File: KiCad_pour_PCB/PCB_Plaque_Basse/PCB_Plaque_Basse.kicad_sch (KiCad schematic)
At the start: 9 parts

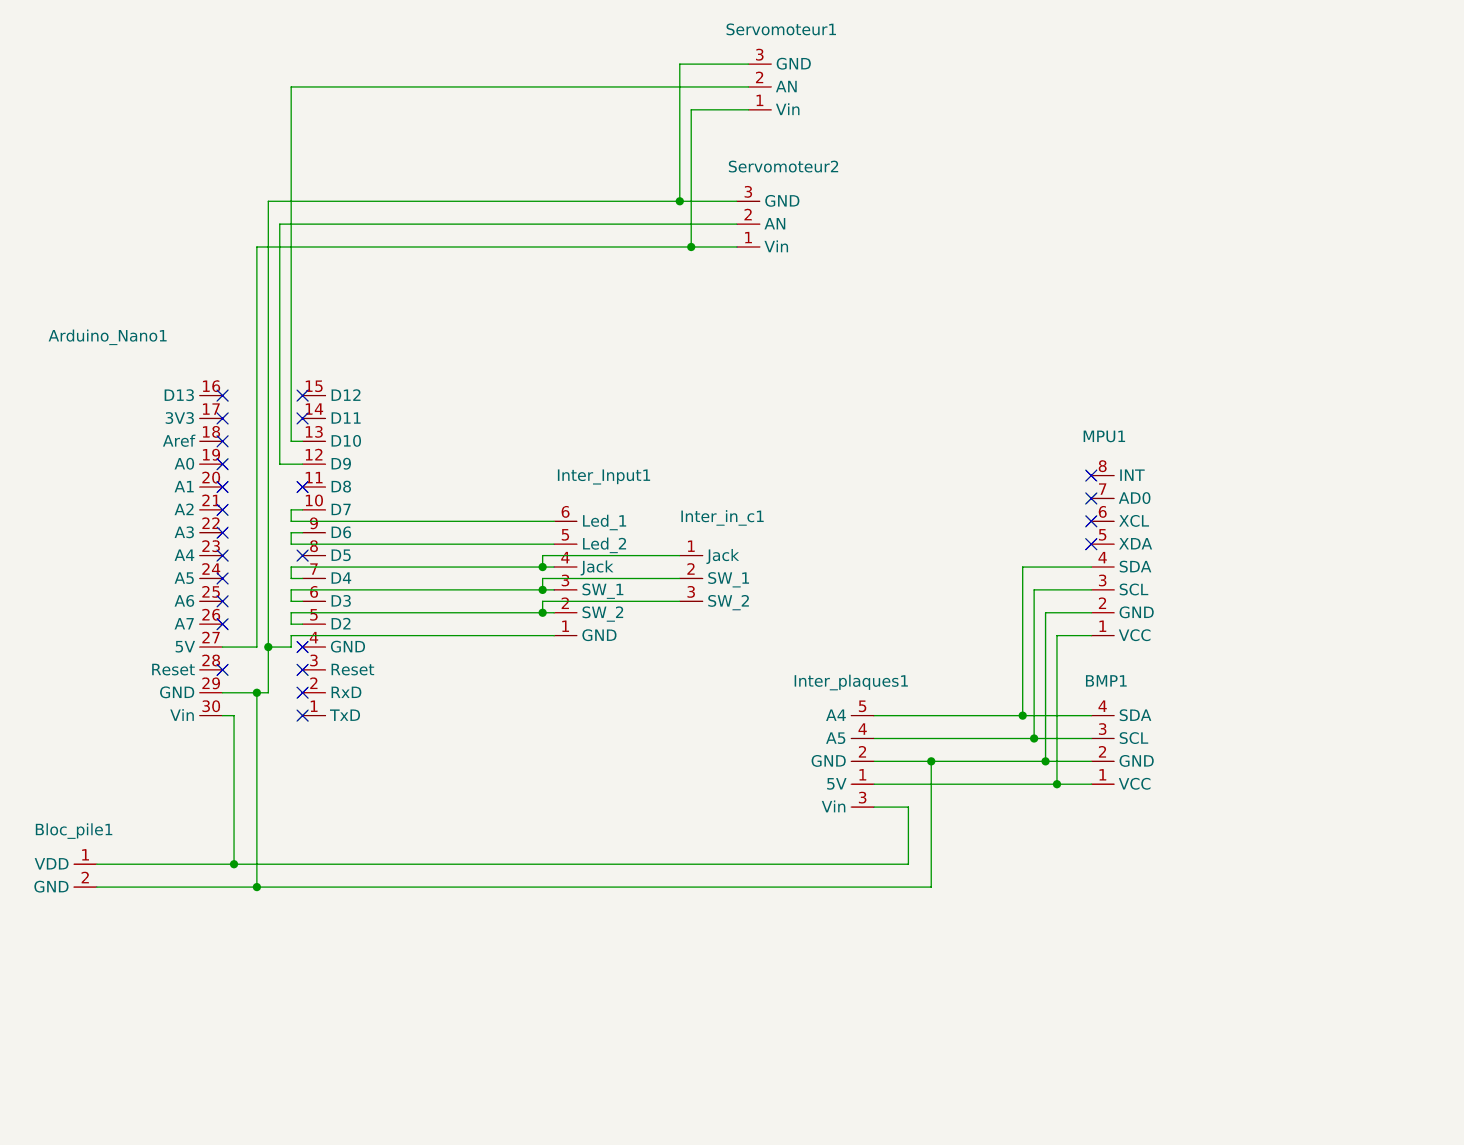
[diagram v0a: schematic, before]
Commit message: Avancement carte PCB
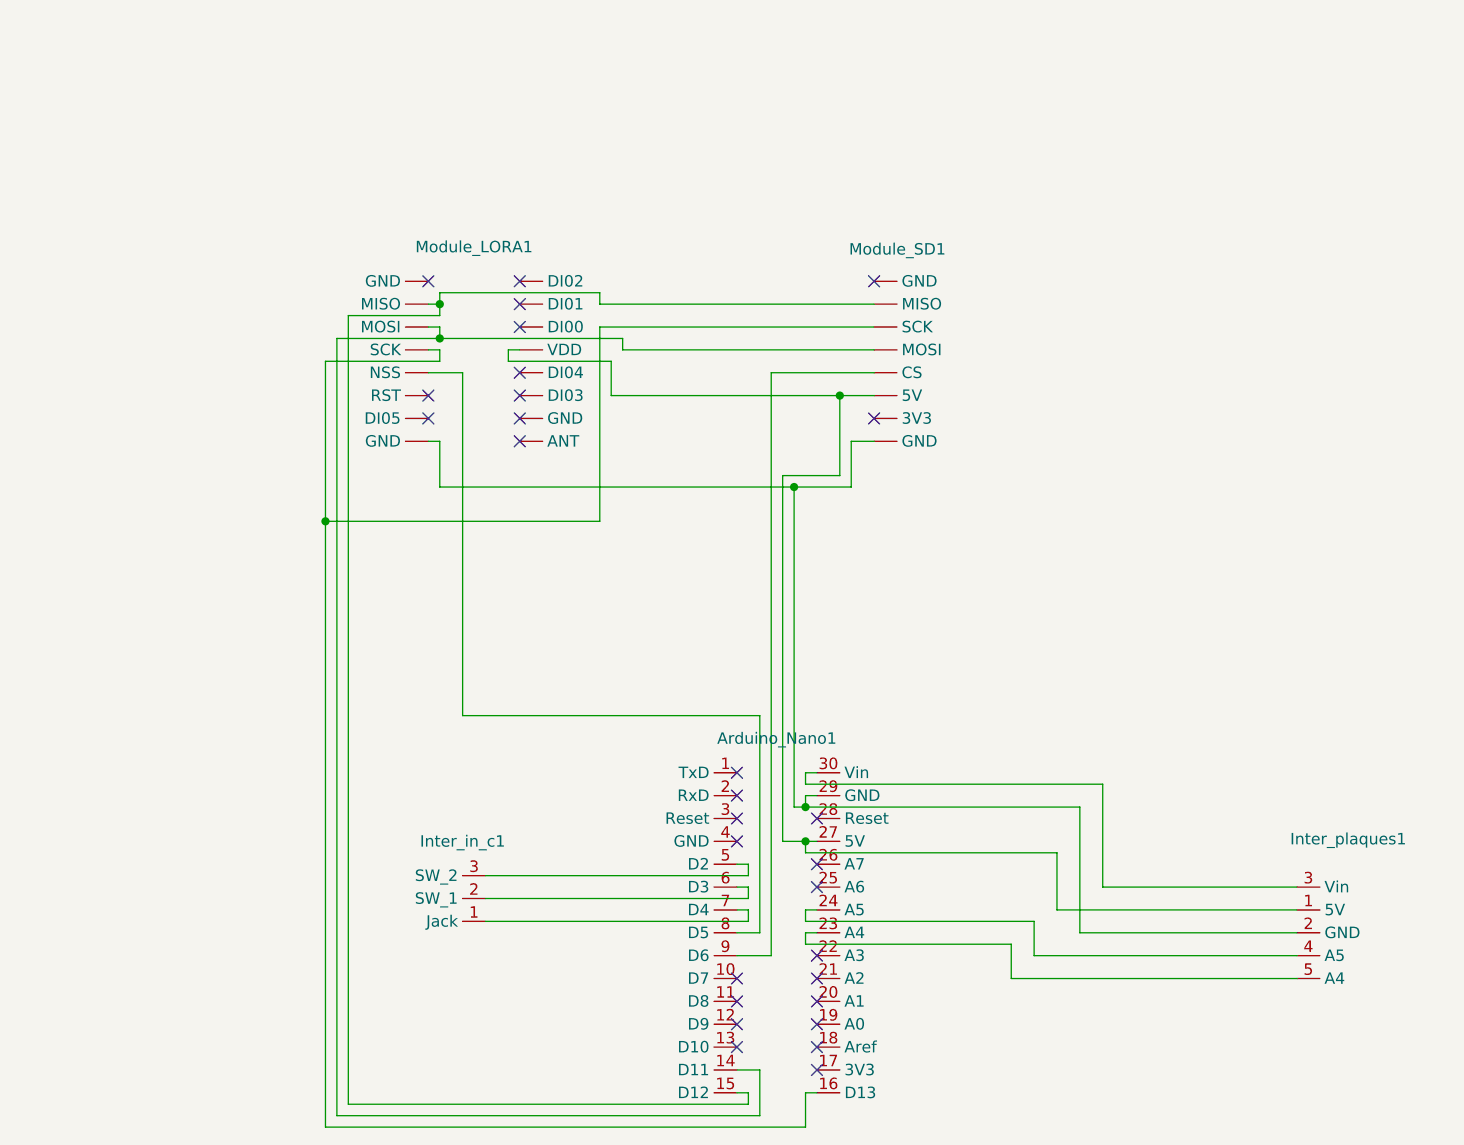
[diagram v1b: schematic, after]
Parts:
- removed BMP1: ~, INSARIANNE_Lib:BMP180, symbol INSARIANNE_Lib:BMP180
- removed Bloc_pile1: ~, Connector_PinHeader_1.00mm:PinHeader_1x02_P1.00mm_Vertical, symbol INSARIANNE_Lib:Bloc_pile
- removed Inter_Input1: ~, Connector_PinHeader_1.00mm:PinHeader_1x06_P1.00mm_Vertical, symbol INSARIANNE_Lib:Interface_input
- removed MPU1: ~, INSARIANNE_Lib:MPU6050, symbol INSARIANNE_Lib:MPU6050
- removed Servomoteur1, Servomoteur2: ~, Connector_PinHeader_1.00mm:PinHeader_1x03_P1.00mm_Vertical, symbol INSARIANNE_Lib:Servomoteur
- added Module_LORA1: ~, symbol INSARIANNE_Lib:Module_LORA
- added Module_SD1: ~, symbol INSARIANNE_Lib:Module_SD
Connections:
- net at Inter_plaques1.1 (5V): now also Arduino_Nano1.27 (5V), Module_LORA1. (VDD), Module_SD1. (SCK)
- net at Arduino_Nano1.29 (GND), Inter_plaques1.2 (GND): now also Module_LORA1. (VDD), Module_SD1. (SCK)
- net at Inter_plaques1.4 (A5): now also Arduino_Nano1.24 (A5)
- net at Inter_plaques1.5 (A4): now also Arduino_Nano1.23 (A4)
- net at Arduino_Nano1.14 (D11): now also Module_LORA1. (VDD), Module_SD1. (SCK)
- net at Arduino_Nano1.15 (D12): now also Module_LORA1. (VDD), Module_SD1. (SCK)
- net at Arduino_Nano1.16 (D13): now also Module_LORA1. (VDD), Module_SD1. (SCK)
- net at Arduino_Nano1.8 (D5): now also Module_LORA1. (VDD)
- net at Arduino_Nano1.9 (D6): now also Module_SD1. (SCK)
- no-connect marks 24 -> 29
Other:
- company: INS'AERO - PÔLE TECHNIQUE - INSA CVL -> (none)
- title: INSARIANNE1 Haute - v3 -> (none)
